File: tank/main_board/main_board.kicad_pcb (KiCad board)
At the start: 2 copper layers, 72.1 x 61.5 mm, 43 parts, among them J1 Encoder0, J10 PowerMotor, J11 M0, J12 M1, J13 M2, J14 Spk, J15 LEDs, J16 SigOut, J2 Encoder1, J3 Encoder2, J4 Encoder3, J5 Programming Header, J6 Bump0, J7 Bump1, J8 PowerOut, J9 PowerIn, U1 L7805, U2 ATMEGA328P-PU, U3 SN74HC595, U4 L293D, U5 L293D, Y1 Crystal

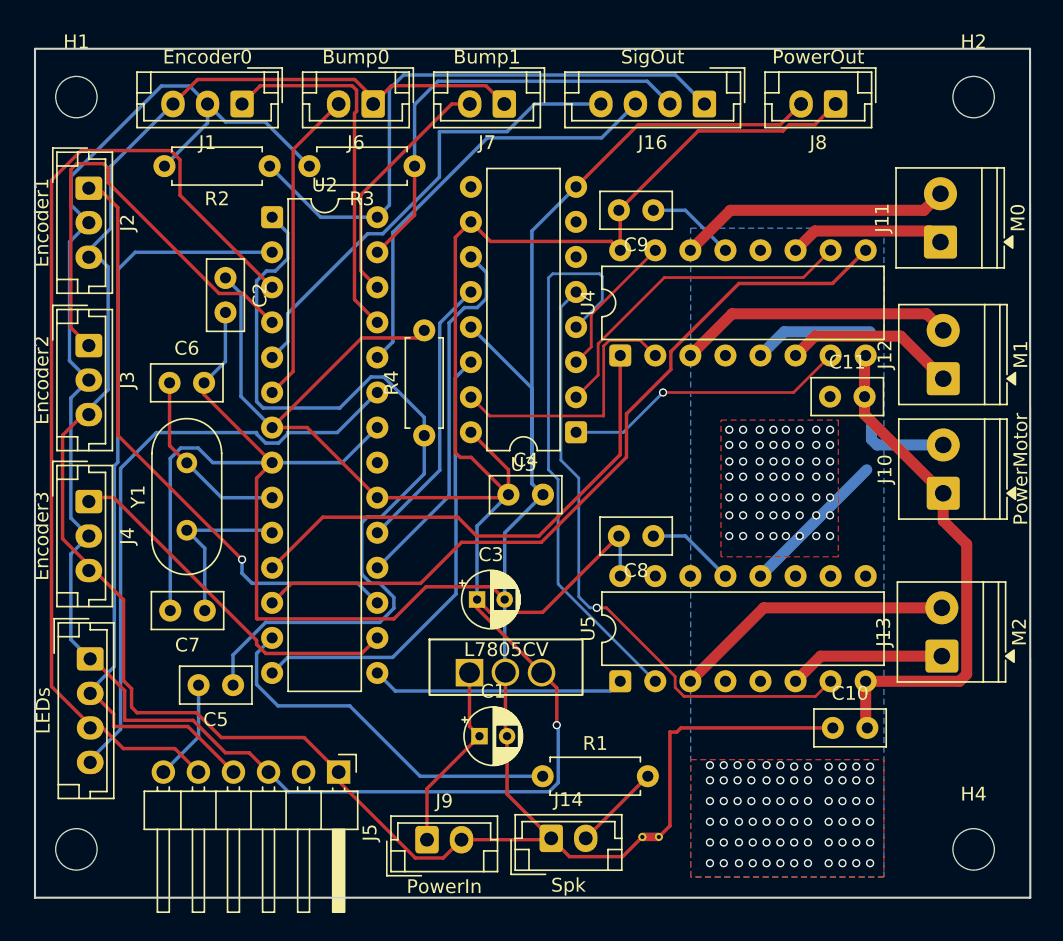
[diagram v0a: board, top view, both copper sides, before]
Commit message: IR Camera v0.2
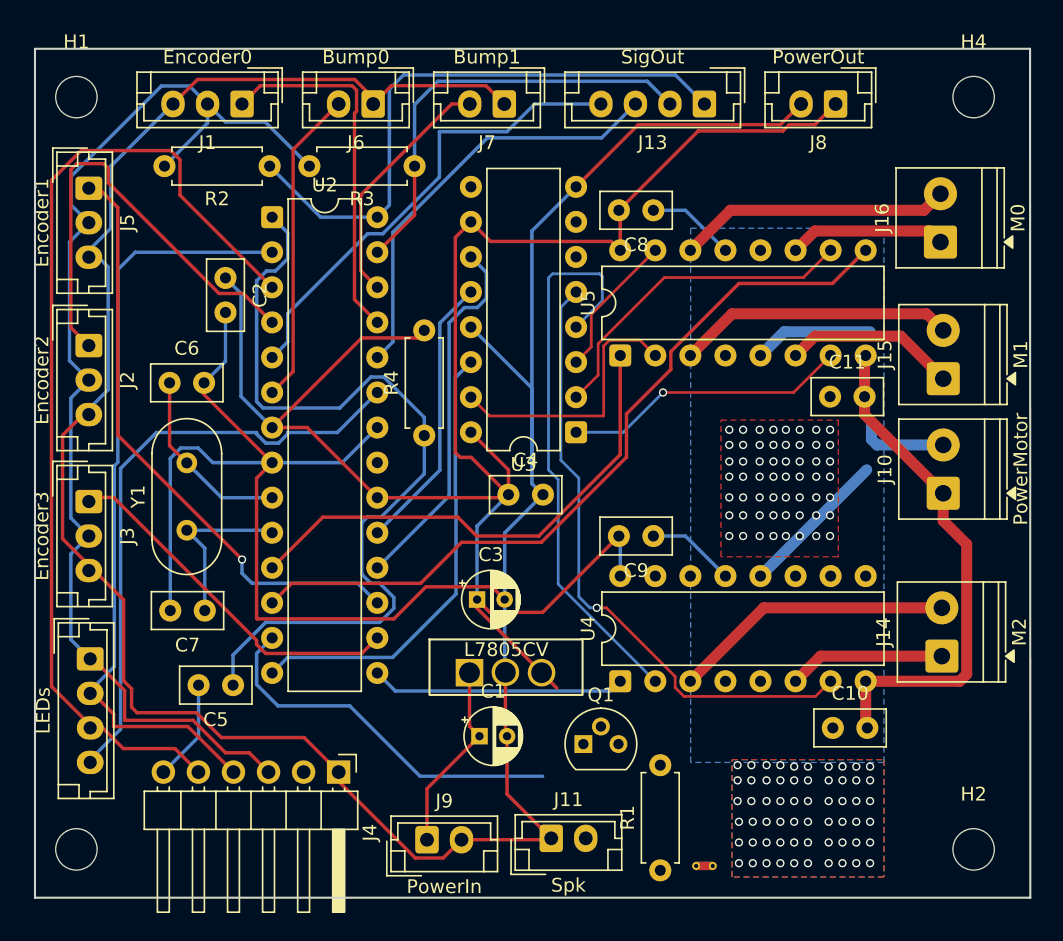
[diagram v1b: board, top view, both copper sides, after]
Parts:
- removed G***: LOGO, custom:Tank
- added Q1: NPN, Package_TO_SOT_THT:TO-92, F.Cu at (130.7, 123.4)
- moved R1 10.9 mm to (136.3, 132.5), turned to 90 degrees
- moved NT1 4.43 mm to (140.1, 132.2)
- renumbered C9 to C8, C8 to C9, H4 to H2, H2 to H4, J14 to J11, J15 to J12, J16 to J13, J13 to J14, J12 to J15, J11 to J16, J3 to J2, J4 to J3, J5 to J4, J2 to J5, U5 to U4, U4 to U5
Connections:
- J11 pad 2: SPK -> Net-(J11-Pin_2)
- R1 pad 1: Net-(U2-(PCINT23/AIN1)PD7) -> SPK
- R1 pad 2: SPK -> Net-(Q1-B)
- U2 pad 13: Net-(U2-(PCINT23/AIN1)PD7) -> SPK
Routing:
- net 4.5V: track 253.6 -> 224.8 mm, vias 1 -> 0
- net Net-(U2-(PCINT23/AIN1)PD7): track 27.3 -> 0.00 mm
- net SPK: track 6.36 -> 27.3 mm
- net Gm: track 58.6 -> 38.8 mm, vias 128 -> 116
- net GND: track 275.0 -> 267.2 mm
